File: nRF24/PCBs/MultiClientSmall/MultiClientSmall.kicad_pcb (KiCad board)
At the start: 2 copper layers, 38 x 38 mm, 16 parts, among them M1 TP4056, SW1 SW_Push_Dual, U1 NRF24L01, U2 ATtiny84, U3 MCP1700x-330, U4 BH1750, U5 AM312

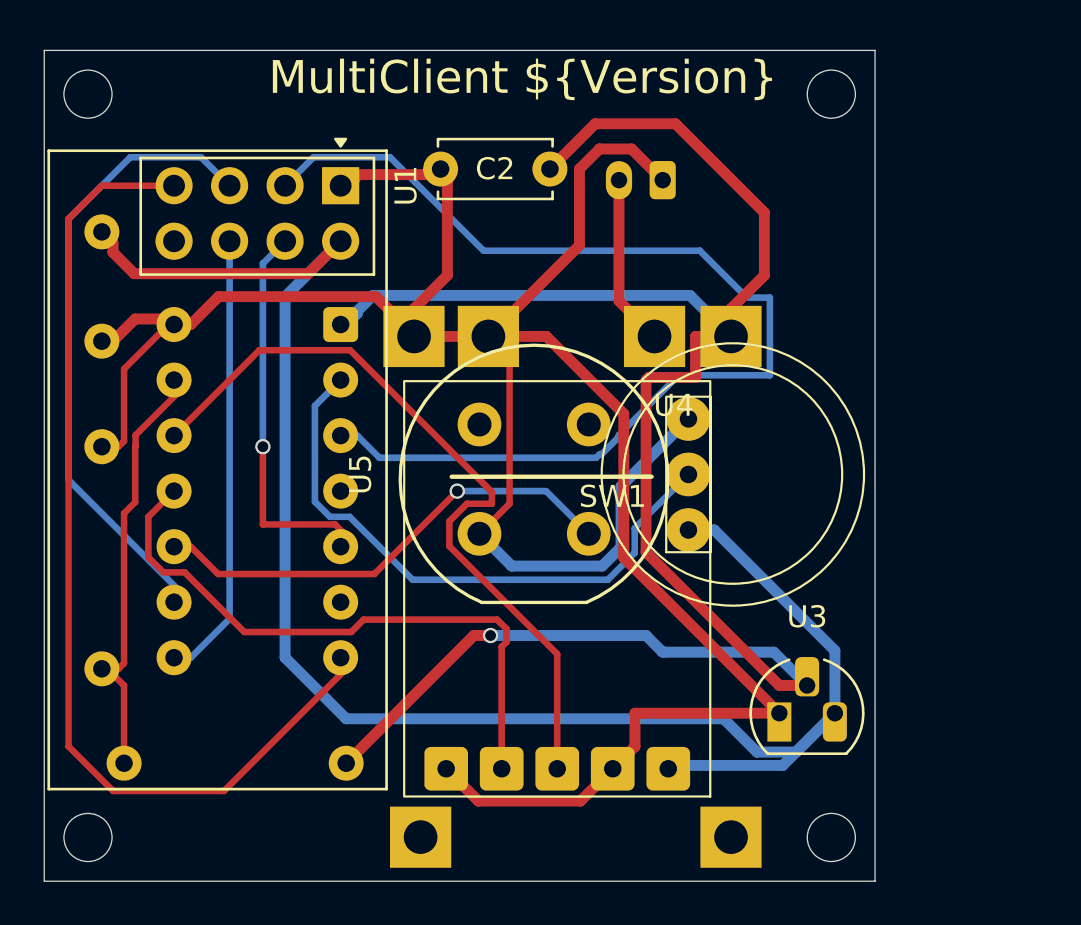
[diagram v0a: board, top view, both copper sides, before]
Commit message: Production Version of nRF24 Multi Client Small
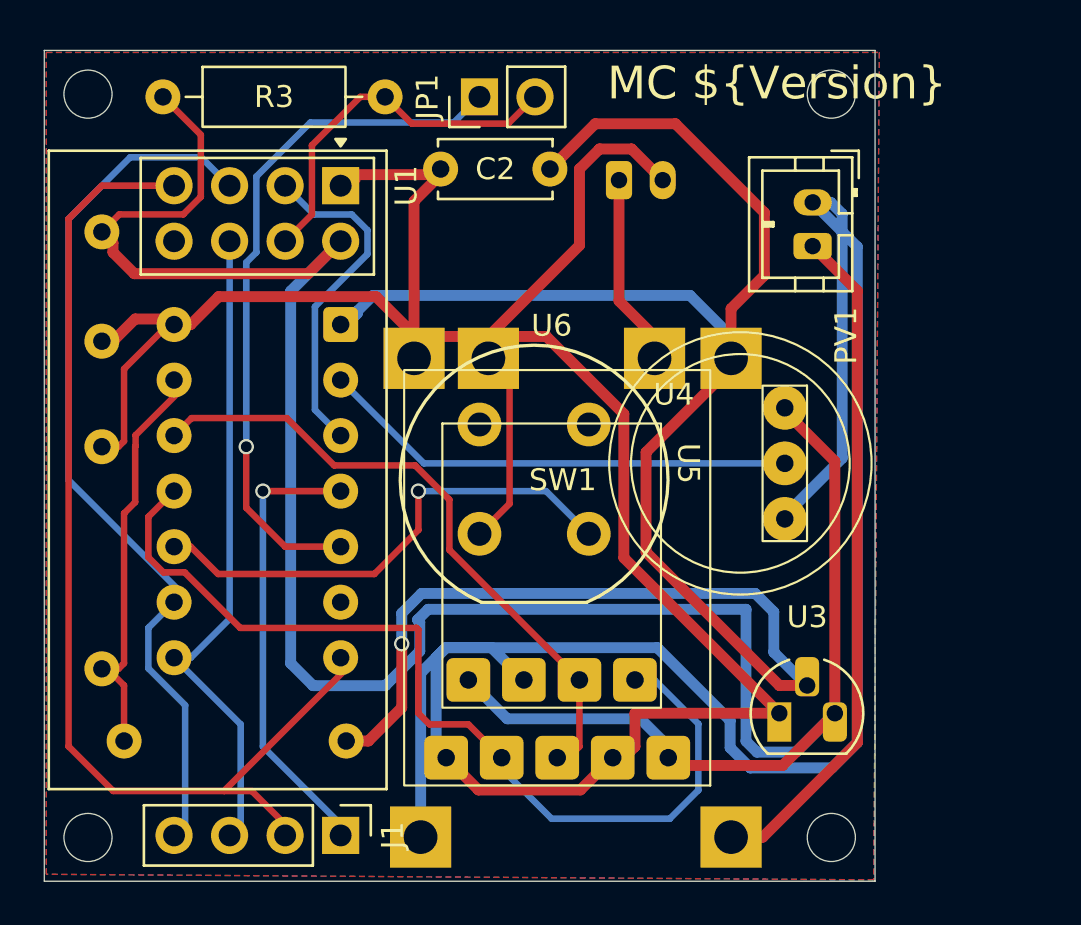
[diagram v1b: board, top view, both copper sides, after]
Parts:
- added J1: Prog, Connector_PinHeader_2.54mm:PinHeader_1x04_P2.54mm_Vertical, F.Cu at (130.6, 136.9)
- added JP1: CSN, Connector_PinHeader_2.54mm:PinHeader_1x02_P2.54mm_Vertical, F.Cu at (136.9, 103.1)
- added PV1: 6V, hagego:JST_PH_1x02_P2.00, F.Cu at (152.1, 108.0)
- added R3: 1M, Resistor_THT:R_Axial_DIN0207_L6.3mm_D2.5mm_P10.16mm_Horizontal, F.Cu at (122.4, 103.1)
- added U6: BME280, hagego:BME280, F.Cu at (140.2, 131.1)
- Bat1: renamed from BT1; footprint Connector_JST:JST_PH_B2B-PH-K_1x02_P2.00mm_Vertical -> hagego:JST_PH_1x02_P2.00
- M1: footprint KiCad Library:TP4056-18650 -> hagego:TP4056-18650
- SW1: value SW_Push_Dual -> Button
- moved R1 1.02 mm to (130.8, 132.6)
- moved U5 0.84 mm to (149.0, 119.9), turned to -90 degrees
- moved U4 0.51 mm to (140.5, 134.6)
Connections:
- net Net-(BT1-+) renamed +3V7
- net Net-(U1-MISO) renamed /MOSI
- net Net-(U1-MOSI) renamed /MISO
- net Net-(U1-SCK) renamed /SCK
- net Net-(U2-PA1) renamed /SCL
- net Net-(U2-PA2) renamed /SDA
- Bat1 pad 2: /GND -> GND
- C1 pad 1: /GND -> GND
- C2 pad 1: /GND -> GND
- M1 pad 1: unconnected-(M1-In+-Pad1) -> +6V
- M1 pad 2: unconnected-(M1-In--Pad2) -> GND
- M1 pad 4: /GND -> GND
- M1 pad 6: /GND -> GND
- R2 pad 2: /GND -> GND
- SW1 pad 3: /GND -> GND
- U1 pad 1: /GND -> GND
- U1 pad 4: Net-(U1-~{CSN}) -> Net-(JP1-B)
- U2 pad 14: /GND -> GND
- U2 pad 4: unconnected-(U2-~{RESET}/PB3-Pad4) -> Net-(J1-Pin_1)
- U2 pad 5: Net-(U1-~{CSN}) -> Net-(JP1-A)
- U3 pad 1: /GND -> GND
- U4 pad 2: /GND -> GND
- U4 pad 5: /GND -> GND
- U5 pad 3: /GND -> GND
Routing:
- net GND: track 0.00 -> 190.8 mm
- net /GND: track 122.7 -> 0.00 mm
- net Net-(U1-CE): track 50.6 -> 15.5 mm
- net Net-(JP1-A): track 0.00 -> 32.1 mm, vias 0 -> 1
- net /VCC: track 81.6 -> 113.4 mm
- net +6V: track 0.00 -> 31.1 mm
- net Net-(J1-Pin_1): track 0.00 -> 20.8 mm, vias 0 -> 1
- net Net-(U1-~{CSN}): track 18.0 -> 0.00 mm, vias 1 -> 0
- net Net-(JP1-B): track 0.00 -> 17.0 mm
- net /SDA: track 28.2 -> 43.5 mm
- net /SCK: track 28.8 -> 40.9 mm
- net /MISO: track 20.5 -> 30.1 mm
- net /SCL: track 35.0 -> 29.5 mm
- net Net-(U2-XTAL1/PB0): track 27.3 -> 21.9 mm
- net /MOSI: track 46.1 -> 50.0 mm
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- added copper zone on B.Cu, net GND
- added copper zone on F.Cu, net GND
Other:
- board text added: "MC ${Version}"
- board text removed: "MultiClient ${Version}"
